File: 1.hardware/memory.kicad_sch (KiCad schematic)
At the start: 2 parts, among them IC1 IS42S32800J-6TLI, U2 NC_IS42S16400J-xC

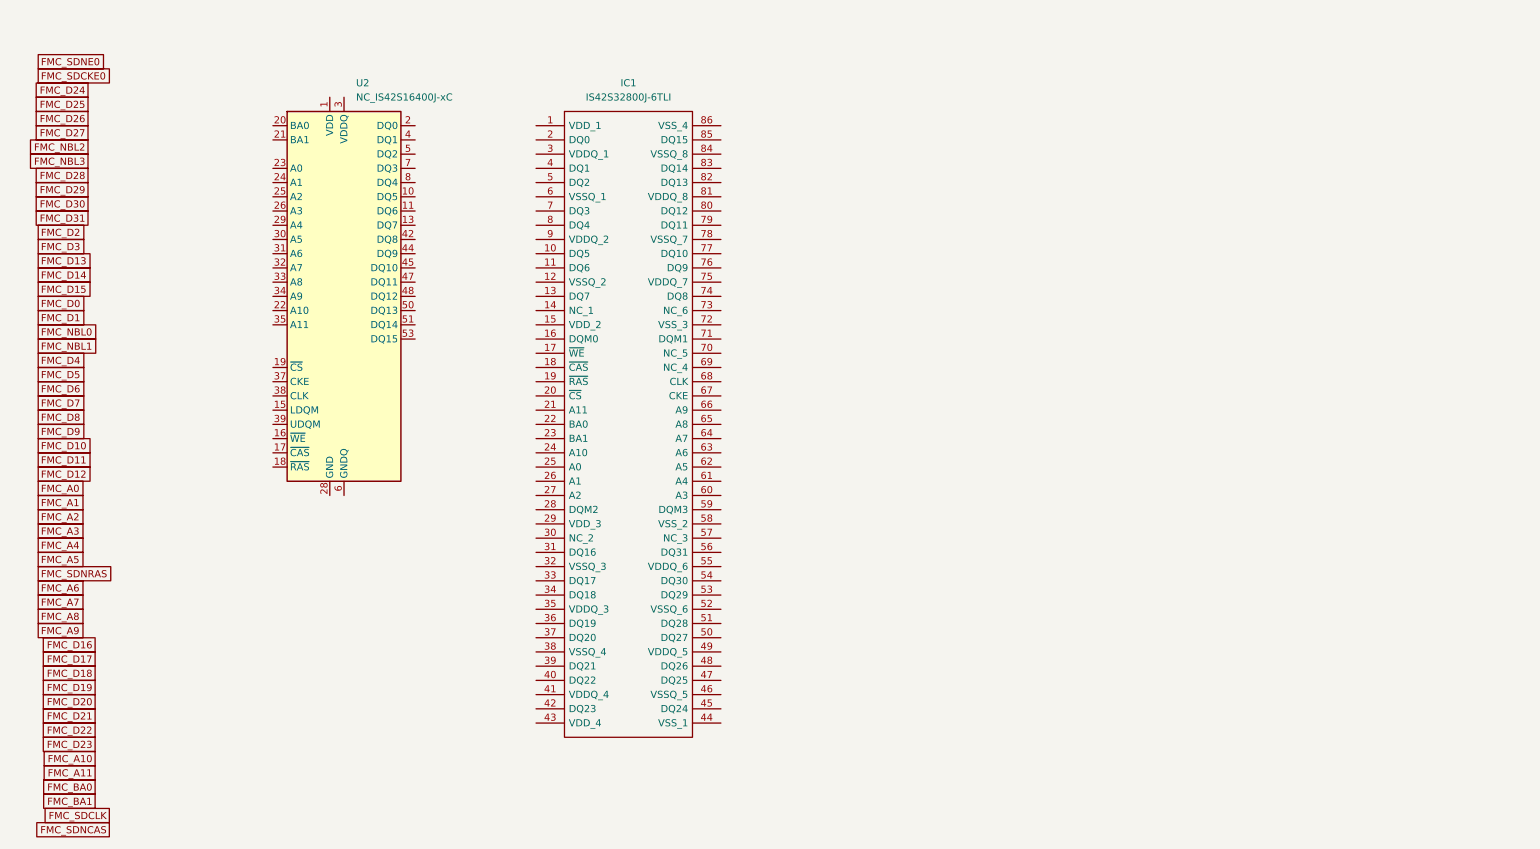
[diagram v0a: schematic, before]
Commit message: 중간 저장2
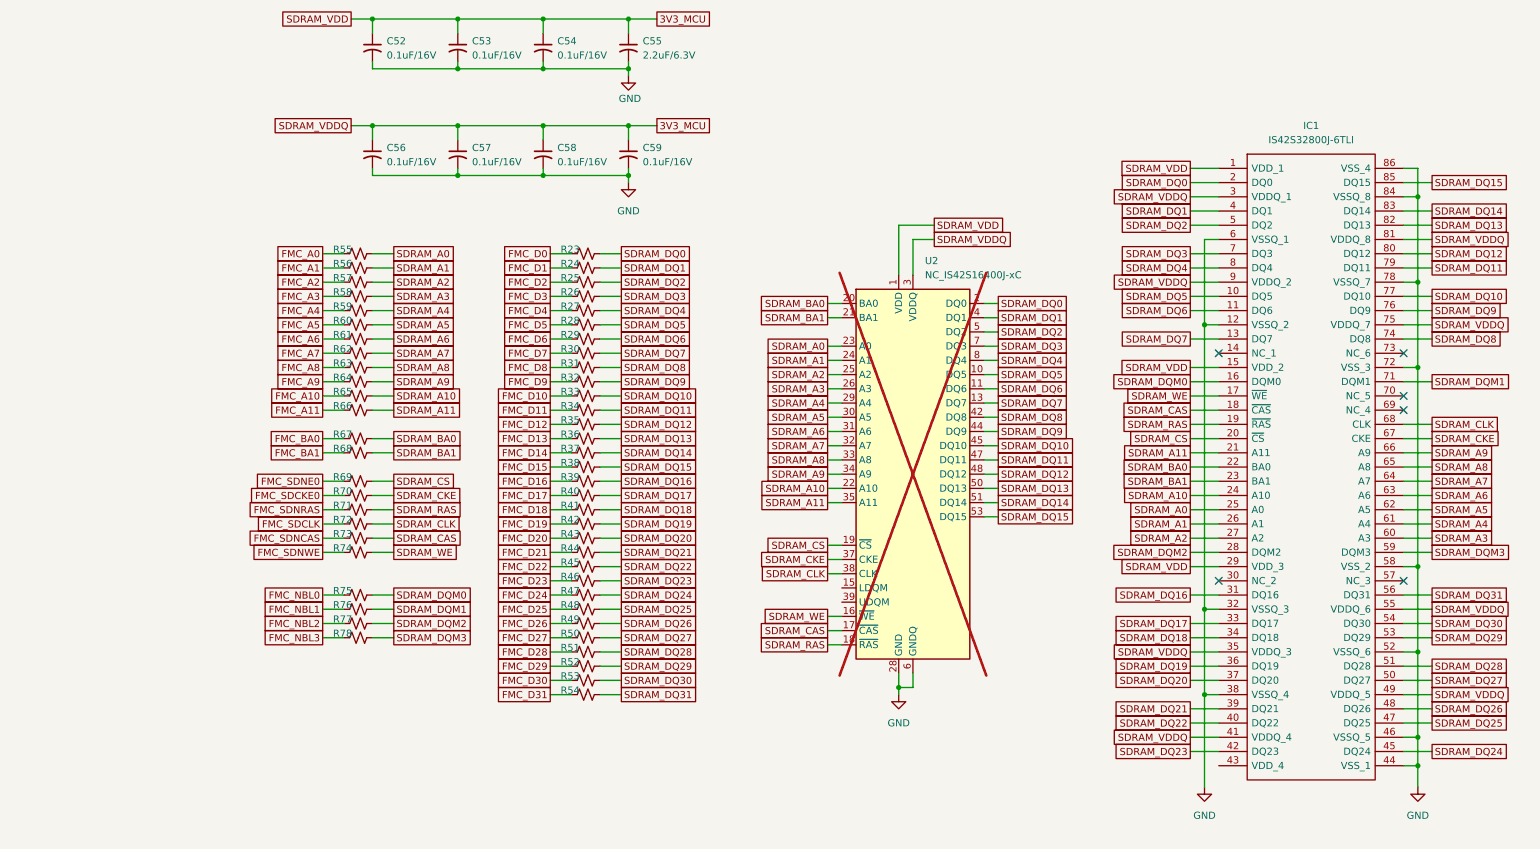
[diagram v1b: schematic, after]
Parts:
- added C52, C53, C54, C56, C57, C58, C59: 0.1uF/16V, Capacitor_SMD:C_0402_1005Metric, symbol Device:C_Small_US
- added C55: 2.2uF/6.3V, Capacitor_SMD:C_0603_1608Metric, symbol Device:C_Small_US
- added R23, R24, R25, R26, R27, R28, R29, R30, R31, R32, R33, R34, R35, R36, R37, R38, R39, R40, R41, R42, R43, R44, R45, R46, R47, R48, R49, R50, R51, R52, R53, R54, R55, R56, R57, R58, R59, R60, R61, R62, R63, R64, R65, R66, R67, R68, R69, R70, R71, R72, R73, R74, R75, R76, R77, R78: 33R/0.063w, symbol Device:R_Small_US
- U2: now not fitted; now left out of the parts list
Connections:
- net FMC_A0: now also R55.1
- net FMC_A1: now also R56.1
- net FMC_A10: now also R65.1
- net FMC_A11: now also R66.1
- net FMC_A2: now also R57.1
- net FMC_A3: now also R58.1
- net FMC_A4: now also R59.1
- net FMC_A5: now also R60.1
- net FMC_A6: now also R61.1
- net FMC_A7: now also R62.1
- net FMC_A8: now also R63.1
- net FMC_A9: now also R64.1
- net FMC_BA0: now also R67.1
- net FMC_BA1: now also R68.1
- net FMC_D0: now also R23.1
- net FMC_D1: now also R24.1
- net FMC_D10: now also R33.1
- net FMC_D11: now also R34.1
- net FMC_D12: now also R35.1
- net FMC_D13: now also R36.1
- net FMC_D14: now also R37.1
- net FMC_D15: now also R38.1
- net FMC_D16: now also R39.1
- net FMC_D17: now also R40.1
- net FMC_D18: now also R41.1
- net FMC_D19: now also R42.1
- net FMC_D2: now also R25.1
- net FMC_D20: now also R43.1
- net FMC_D21: now also R44.1
- net FMC_D22: now also R45.1
- net FMC_D23: now also R46.1
- net FMC_D24: now also R47.1
- net FMC_D25: now also R48.1
- net FMC_D26: now also R49.1
- net FMC_D27: now also R50.1
- net FMC_D28: now also R51.1
- net FMC_D29: now also R52.1
- net FMC_D3: now also R26.1
- net FMC_D30: now also R53.1
- net FMC_D31: now also R54.1
- net FMC_D4: now also R27.1
- net FMC_D5: now also R28.1
- net FMC_D6: now also R29.1
- net FMC_D7: now also R30.1
- net FMC_D8: now also R31.1
- net FMC_D9: now also R32.1
- net FMC_NBL0: now also R75.1
- net FMC_NBL1: now also R76.1
- net FMC_NBL2: now also R77.1
- net FMC_NBL3: now also R78.1
- net FMC_SDCKE0: now also R70.1
- net FMC_SDCLK: now also R72.1
- net FMC_SDNCAS: now also R73.1
- net FMC_SDNE0: now also R69.1
- net FMC_SDNRAS: now also R71.1
- net 3V3_MCU: now reaches U2.1 (VDD), U2.14 (VDD), U2.27 (VDD)
- net 3V3_MCU: now also IC1.1 (VDD_1), IC1.15 (VDD_2), IC1.29 (VDD_3), IC1.3 (VDDQ_1), IC1.35 (VDDQ_3), IC1.41 (VDDQ_4), IC1.49 (VDDQ_5), IC1.55 (VDDQ_6), IC1.75 (VDDQ_7), IC1.81 (VDDQ_8), IC1.9 (VDDQ_2), U2.3 (VDDQ), U2.43 (VDDQ), U2.49 (VDDQ), U2.9 (VDDQ), C52.1, C53.1, C54.1, C55.1, C56.1, C57.1, C58.1, C59.1
- net SDRAM_DQ5: now reaches U2.10 (DQ5)
- net SDRAM_DQ5: now also IC1.10 (DQ5), R28.2
- net SDRAM_DQ6: now reaches U2.11 (DQ6)
- net SDRAM_DQ6: now also IC1.11 (DQ6), R29.2
- net GND: now reaches U2.12 (GNDQ), U2.46 (GNDQ), U2.52 (GNDQ), U2.6 (GNDQ)
- net GND: now also IC1.12 (VSSQ_2), IC1.32 (VSSQ_3), IC1.38 (VSSQ_4), IC1.44 (VSS_1), IC1.46 (VSSQ_5), IC1.52 (VSSQ_6), IC1.58 (VSS_2), IC1.6 (VSSQ_1), IC1.72 (VSS_3), IC1.78 (VSSQ_7), IC1.84 (VSSQ_8), IC1.86 (VSS_4), U2.28 (GND), U2.41 (GND), U2.54 (GND), C52.2, C53.2, C54.2, C55.2, C56.2, C57.2, C58.2, C59.2
- net SDRAM_DQ7: now reaches U2.13 (DQ7)
- net SDRAM_DQ7: now also IC1.13 (DQ7), R30.2
- net SDRAM_WE: now reaches U2.16 (~{WE})
- net SDRAM_WE: now also IC1.17 (~{WE}), R74.2
- net SDRAM_CAS: now reaches U2.17 (~{CAS})
- net SDRAM_CAS: now also IC1.18 (~{CAS}), R73.2
- net SDRAM_RAS: now reaches U2.18 (~{RAS})
- net SDRAM_RAS: now also IC1.19 (~{RAS}), R71.2
- net SDRAM_CS: now reaches U2.19 (~{CS})
- net SDRAM_CS: now also IC1.20 (~{CS}), R69.2
- net SDRAM_DQ0: now reaches U2.2 (DQ0)
- net SDRAM_DQ0: now also IC1.2 (DQ0), R23.2
- net SDRAM_BA0: now reaches U2.20 (BA0)
- net SDRAM_BA0: now also IC1.22 (BA0), R67.2
- net SDRAM_BA1: now reaches U2.21 (BA1)
- net SDRAM_BA1: now also IC1.23 (BA1), R68.2
- net SDRAM_A10: now reaches U2.22 (A10)
- net SDRAM_A10: now also IC1.24 (A10), R65.2
- net SDRAM_A0: now reaches U2.23 (A0)
- net SDRAM_A0: now also IC1.25 (A0), R55.2
- net SDRAM_A1: now reaches U2.24 (A1)
- net SDRAM_A1: now also IC1.26 (A1), R56.2
- net SDRAM_A2: now reaches U2.25 (A2)
- net SDRAM_A2: now also IC1.27 (A2), R57.2
- net SDRAM_A3: now reaches U2.26 (A3)
- net SDRAM_A3: now also IC1.60 (A3), R58.2
- net SDRAM_A4: now reaches U2.29 (A4)
- net SDRAM_A4: now also IC1.61 (A4), R59.2
- net SDRAM_A5: now reaches U2.30 (A5)
- net SDRAM_A5: now also IC1.62 (A5), R60.2
- net SDRAM_A6: now reaches U2.31 (A6)
- net SDRAM_A6: now also IC1.63 (A6), R61.2
- net SDRAM_A7: now reaches U2.32 (A7)
- net SDRAM_A7: now also IC1.64 (A7), R62.2
- net SDRAM_A8: now reaches U2.33 (A8)
- net SDRAM_A8: now also IC1.65 (A8), R63.2
- net SDRAM_A9: now reaches U2.34 (A9)
- net SDRAM_A9: now also IC1.66 (A9), R64.2
- net SDRAM_A11: now reaches U2.35 (A11)
- net SDRAM_A11: now also IC1.21 (A11), R66.2
- net SDRAM_CKE: now reaches U2.37 (CKE)
- net SDRAM_CKE: now also IC1.67 (CKE), R70.2
- net SDRAM_CLK: now reaches U2.38 (CLK)
- net SDRAM_CLK: now also IC1.68 (CLK), R72.2
- net SDRAM_DQ1: now reaches U2.4 (DQ1)
- net SDRAM_DQ1: now also IC1.4 (DQ1), R24.2
- net SDRAM_DQ8: now reaches U2.42 (DQ8)
- net SDRAM_DQ8: now also IC1.74 (DQ8), R31.2
- net SDRAM_DQ9: now reaches U2.44 (DQ9)
- net SDRAM_DQ9: now also IC1.76 (DQ9), R32.2
- net SDRAM_DQ10: now reaches U2.45 (DQ10)
- net SDRAM_DQ10: now also IC1.77 (DQ10), R33.2
- net SDRAM_DQ11: now reaches U2.47 (DQ11)
- net SDRAM_DQ11: now also IC1.79 (DQ11), R34.2
- net SDRAM_DQ12: now reaches U2.48 (DQ12)
- net SDRAM_DQ12: now also IC1.80 (DQ12), R35.2
- net SDRAM_DQ2: now reaches U2.5 (DQ2)
- net SDRAM_DQ2: now also IC1.5 (DQ2), R25.2
- net SDRAM_DQ13: now reaches U2.50 (DQ13)
- net SDRAM_DQ13: now also IC1.82 (DQ13), R36.2
- net SDRAM_DQ14: now reaches U2.51 (DQ14)
- net SDRAM_DQ14: now also IC1.83 (DQ14), R37.2
- net SDRAM_DQ15: now reaches U2.53 (DQ15)
- net SDRAM_DQ15: now also IC1.85 (DQ15), R38.2
- net SDRAM_DQ3: now reaches U2.7 (DQ3)
- net SDRAM_DQ3: now also IC1.7 (DQ3), R26.2
- net SDRAM_DQ4: now reaches U2.8 (DQ4)
- net SDRAM_DQ4: now also IC1.8 (DQ4), R27.2
- net SDRAM_DQM0: now reaches IC1.16 (DQM0)
- net SDRAM_DQM0: now also R75.2
- net SDRAM_DQM2: now reaches IC1.28 (DQM2)
- net SDRAM_DQM2: now also R77.2
- net SDRAM_DQ16: now reaches IC1.31 (DQ16)
- net SDRAM_DQ16: now also R39.2
- net SDRAM_DQ17: now reaches IC1.33 (DQ17)
- net SDRAM_DQ17: now also R40.2
- net SDRAM_DQ18: now reaches IC1.34 (DQ18)
- net SDRAM_DQ18: now also R41.2
- net SDRAM_DQ19: now reaches IC1.36 (DQ19)
- net SDRAM_DQ19: now also R42.2
- net SDRAM_DQ20: now reaches IC1.37 (DQ20)
- net SDRAM_DQ20: now also R43.2
- net SDRAM_DQ21: now reaches IC1.39 (DQ21)
- net SDRAM_DQ21: now also R44.2
- net SDRAM_DQ22: now reaches IC1.40 (DQ22)
- net SDRAM_DQ22: now also R45.2
- net SDRAM_DQ23: now reaches IC1.42 (DQ23)
- net SDRAM_DQ23: now also R46.2
- net SDRAM_DQ24: now reaches IC1.45 (DQ24)
- net SDRAM_DQ24: now also R47.2
- net SDRAM_DQ25: now reaches IC1.47 (DQ25)
- net SDRAM_DQ25: now also R48.2
- net SDRAM_DQ26: now reaches IC1.48 (DQ26)
- net SDRAM_DQ26: now also R49.2
- net SDRAM_DQ27: now reaches IC1.50 (DQ27)
- net SDRAM_DQ27: now also R50.2
- net SDRAM_DQ28: now reaches IC1.51 (DQ28)
- net SDRAM_DQ28: now also R51.2
- net SDRAM_DQ29: now reaches IC1.53 (DQ29)
- net SDRAM_DQ29: now also R52.2
- net SDRAM_DQ30: now reaches IC1.54 (DQ30)
- net SDRAM_DQ30: now also R53.2
- net SDRAM_DQ31: now reaches IC1.56 (DQ31)
- net SDRAM_DQ31: now also R54.2
- net SDRAM_DQM3: now reaches IC1.59 (DQM3)
- net SDRAM_DQM3: now also R78.2
- net SDRAM_DQM1: now reaches IC1.71 (DQM1)
- net SDRAM_DQM1: now also R76.2
- new net FMC_SDNWE: R74.1
- no-connect marks 0 -> 6
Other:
- moved on the sheet: IC1
